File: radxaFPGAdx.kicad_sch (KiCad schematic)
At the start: 1 part, among them IC1 GW1NR-LV9QN88C7_I6

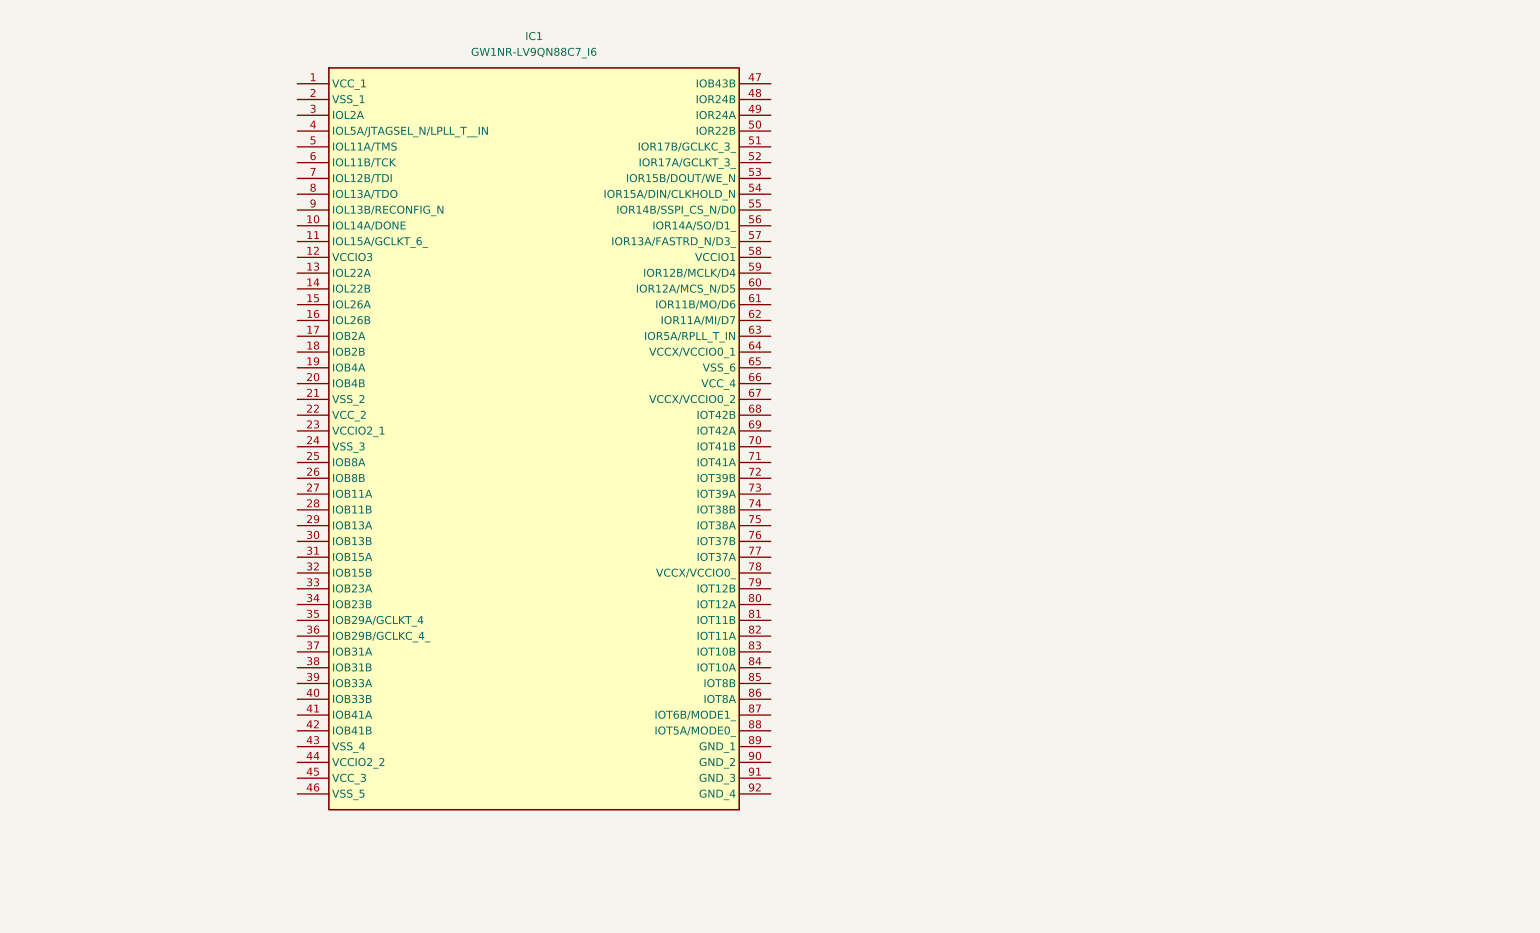
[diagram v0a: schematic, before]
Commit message: Researched and added components: USB, ATmega, Power Mux, Header
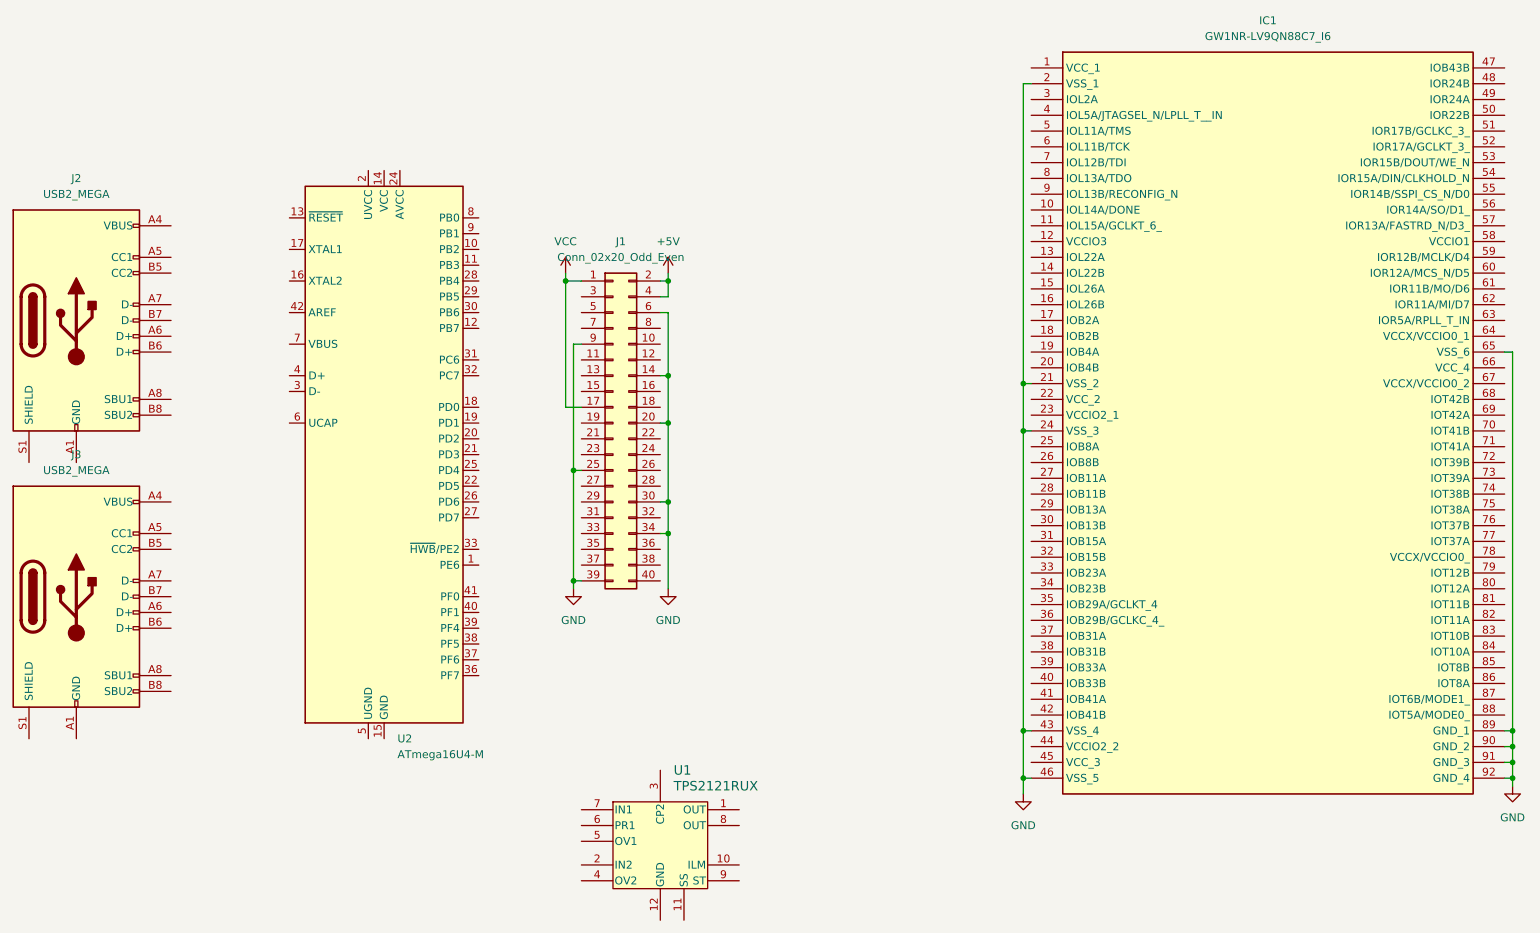
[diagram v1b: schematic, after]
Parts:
- added J1: Conn_02x20_Odd_Even, Connector_PinSocket_2.54mm:PinSocket_2x20_P2.54mm_Vertical, symbol Connector_Generic:Conn_02x20_Odd_Even
- added J2, J3: USB2_MEGA, symbol USB-C-USB-2.0-cache:Connector_USB_C_Receptacle_USB2.0
- added U1: TPS2121RUX, RUX0012A, symbol TI_TPS2121:TPS2121RUX
- added U2: ATmega16U4-M, Package_DFN_QFN:QFN-44-1EP_7x7mm_P0.5mm_EP5.2x5.2mm, symbol MCU_Microchip_ATmega:ATmega16U4-M
- IC1: footprint GW1NRLV9QN88C7I6 -> SamacSys_Parts:GW1NRLV9QN88C7I6
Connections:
- net GND: now reaches IC1.2 (VSS_1)
- net GND: now also IC1.21 (VSS_2), IC1.24 (VSS_3), IC1.43 (VSS_4), IC1.46 (VSS_5), IC1.65 (VSS_6), IC1.89 (GND_1), IC1.90 (GND_2), IC1.91 (GND_3), IC1.92 (GND_4), J1.14 (Pin_14), J1.20 (Pin_20), J1.25 (Pin_25), J1.30 (Pin_30), J1.34 (Pin_34), J1.39 (Pin_39), J1.6 (Pin_6), J1.9 (Pin_9), J2.A1 (GND), J2.A12 (GND), J2.B1 (GND), J2.B12 (GND), J3.A1 (GND), J3.A12 (GND), J3.B1 (GND), J3.B12 (GND)
- new net: U2.14 (VCC), U2.34 (VCC)
- new net: U2.15 (GND), U2.23 (GND), U2.35 (GND), U2.43 (GND), U2.45 (GND)
- new net: U2.24 (AVCC), U2.44 (AVCC)
- new net +5V: J1.2 (Pin_2), J1.4 (Pin_4)
- new net VBUS: J2.A4 (VBUS), J2.A9 (VBUS), J2.B4 (VBUS), J2.B9 (VBUS), J3.A4 (VBUS), J3.A9 (VBUS), J3.B4 (VBUS), J3.B9 (VBUS)
- new net VCC: J1.1 (Pin_1), J1.17 (Pin_17)
